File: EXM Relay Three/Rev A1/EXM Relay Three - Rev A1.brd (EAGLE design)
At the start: 80 x 50 mm, 24 parts, among them J1 MSTBA3, J10 MSTBA2, J2 MSTBA3, J3 22-05-7038-03, J4 22-05-7038-03, J5 22-05-7038-03, J6 22-05-7038-03, J7 MSTBA3, J8 22-05-7038-03, J9 22-05-7038-03, K1 MY2, K2 MY2, K3 MY2, T1 EXMACHINA-LOGO-NAME

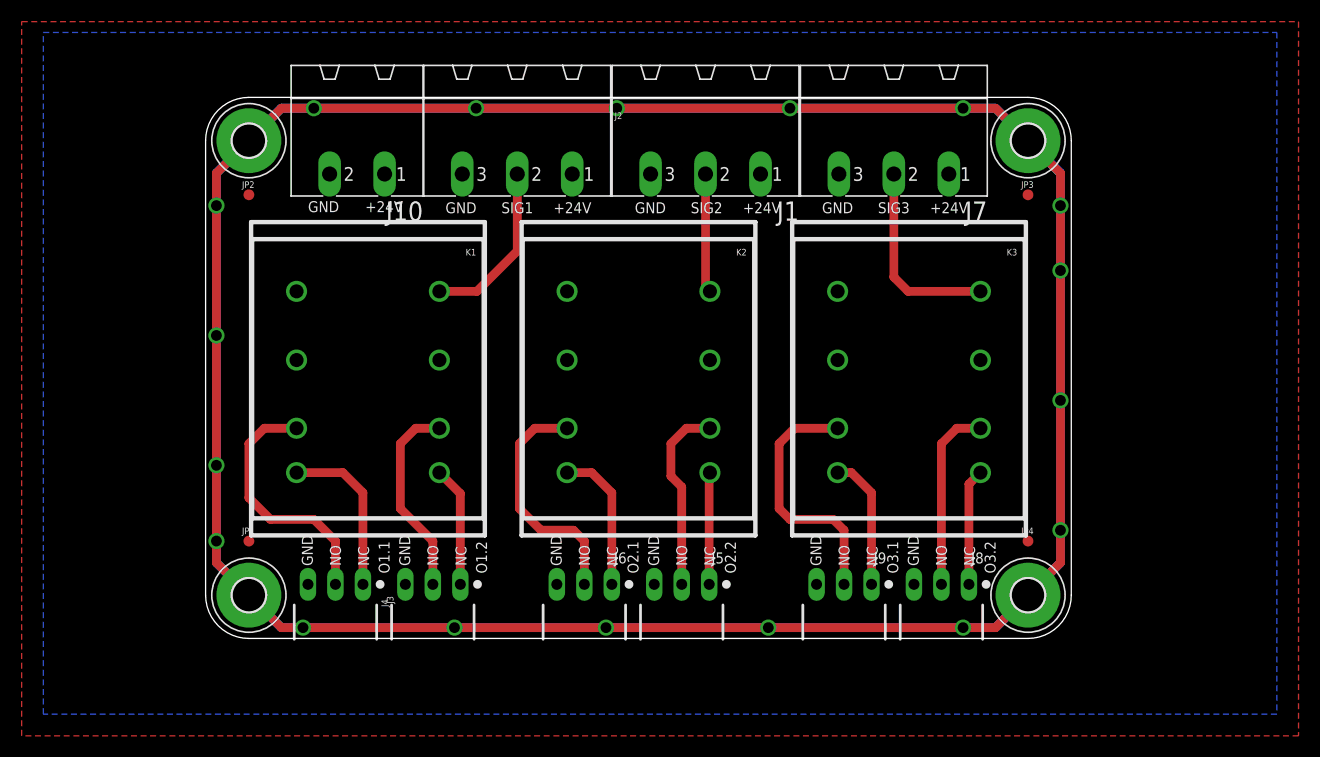
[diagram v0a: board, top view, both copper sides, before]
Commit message: Generate MDP files
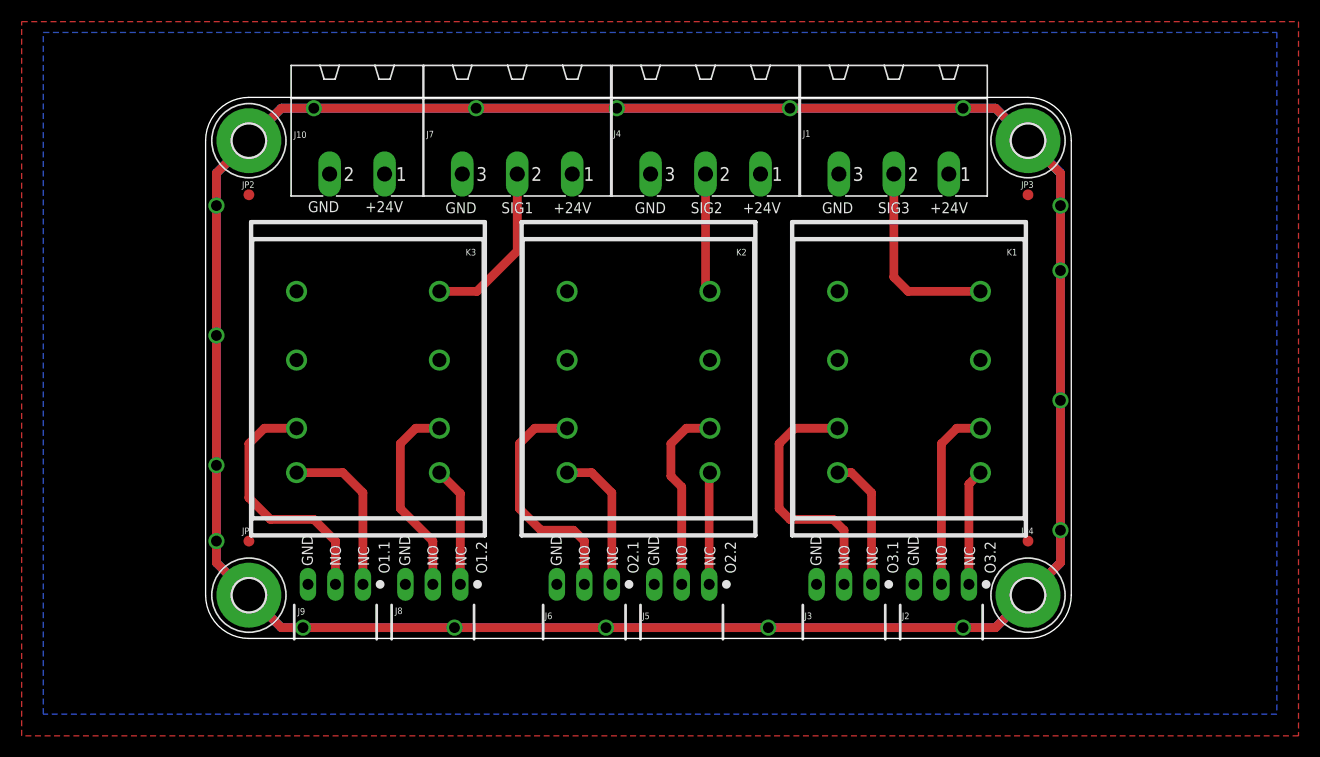
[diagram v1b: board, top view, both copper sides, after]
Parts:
- J2: value MSTBA3 -> 22-05-7038-03; device con-phoenix-508:MSTBA3 -> con-molex:7395-03
- J4: value 22-05-7038-03 -> MSTBA3; device con-molex:7395-03 -> con-phoenix-508:MSTBA3
- moved J2 58.2 mm to (68.0, 5.00), turned to 0 degrees
- moved K1 50.0 mm to (65.0, 24.0)
- moved K3 50.0 mm to (15.0, 24.0)
- moved J4 49.8 mm to (46.2, 48.0), turned to 180 degrees
- moved J3 47.0 mm to (59.0, 5.00)
- moved J8 47.0 mm to (21.0, 5.00)
- moved J9 47.0 mm to (12.0, 5.00)
- moved J7 34.8 mm to (28.8, 48.0)
- moved J1 17.4 mm to (63.6, 48.0)
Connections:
- net +24V: now also J4.1; no longer J2.1
- net SIG1_1_NC: now also J9.1, K3.1; no longer J3.1, K1.1
- net SIG1_1_NO: now also J9.2, K3.5; no longer J3.2, K1.5
- net SIG1_2_NC: now also J8.1, K3.4; no longer J4.1, K1.4
- net SIG1_2_NO: now also J8.2, K3.8; no longer J4.2, K1.8
- net SIG3_1_NC: now also J3.1, K1.1; no longer J9.1, K3.1
- net SIG3_1_NO: now also J3.2, K1.5; no longer J9.2, K3.5
- net SIG3_2_NC: now also J2.1, K1.4; no longer J8.1, K3.4
- net SIG3_2_NO: now also J2.2, K1.8; no longer J8.2, K3.8
- net SIG_IN_1: now also J7.2, K3.14; no longer J2.2, K1.14
- net SIG_IN_2: now also J4.2; no longer J1.2
- net SIG_IN_3: now also J1.2, K1.14; no longer J7.2, K3.14
